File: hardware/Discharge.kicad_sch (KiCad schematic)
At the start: 6 parts, among them Q2 CPH3351

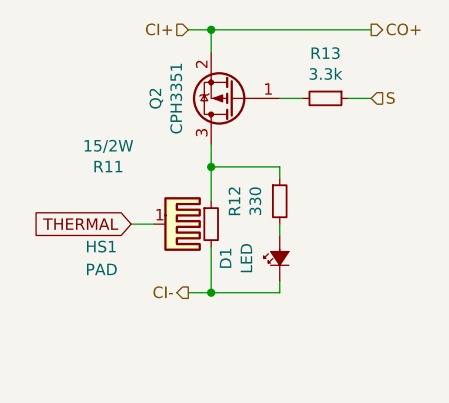
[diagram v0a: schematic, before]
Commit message: finished layout
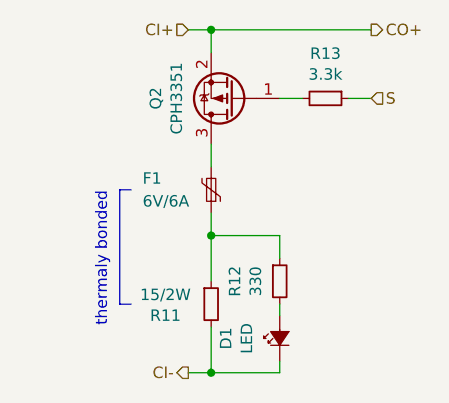
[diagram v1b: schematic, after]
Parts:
- removed HS1: PAD, Connector_Wire:SolderWirePad_1x01_SMD_1x2mm, symbol Mechanical:Heatsink_Pad
- added F1: 6V/6A, Samacsys:1206L075SLYR, symbol 1206l600slwr:1206L600SLWR
- D1: Manufacturer_Part_Number (none) -> 150060SS75000; Mouser Part Number (none) -> 710-150060SS75000; Mouser Price/Stock (none) -> https://www.mouser.pl/ProductDetail/Wurth-Elektronik/150060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
- Q2: Manufacturer_Part_Number (none) -> MMFTP3401; Mouser Part Number (none) -> 637-MMFTP3401; Mouser Price/Stock (none) -> https://www.mouser.pl/ProductDetail/Diotec-Semiconductor/MM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
- R11: footprint Resistor_SMD:R_2512_6332Metric -> Samacsys:RESC6331X80N; Manufacturer_Part_Number (none) -> CRM2512QFW-10R0ELF; Mouser Part Number (none) -> 652-CRM2512QFW-10R0E; Mouser Price/Stock (none) -> https://www.mouser.pl/ProductDetail/Bourns/CRM2512QFW-10R0E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
- R12: Manufacturer_Part_Number (none) -> RT0603FRE07330RL; Mouser Part Number (none) -> 603-RT0603FRE07330RL; Mouser Price/Stock (none) -> https://www.mouser.pl/ProductDetail/YAGEO/RT0603FRE07330RL?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
- R13: Manufacturer_Part_Number (none) -> RT0603FRE073K3L; Mouser Part Number (none) -> 603-RT0603FRE073K3L; Mouser Price/Stock (none) -> https://www.mouser.pl/ProductDetail/YAGEO/RT0603FRE073K3L?q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
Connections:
- net at R11.1, R12.1: now also F1.1; no longer Q2.3 (D)
- new net: F1.2, Q2.3 (D)
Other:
- note added: "thermaly bonded"
- moved on the sheet: D1, R11, R12
